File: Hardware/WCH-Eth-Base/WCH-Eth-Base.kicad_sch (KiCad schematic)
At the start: 1 part, among them J7 Conn_02x32_Counter_Clockwise

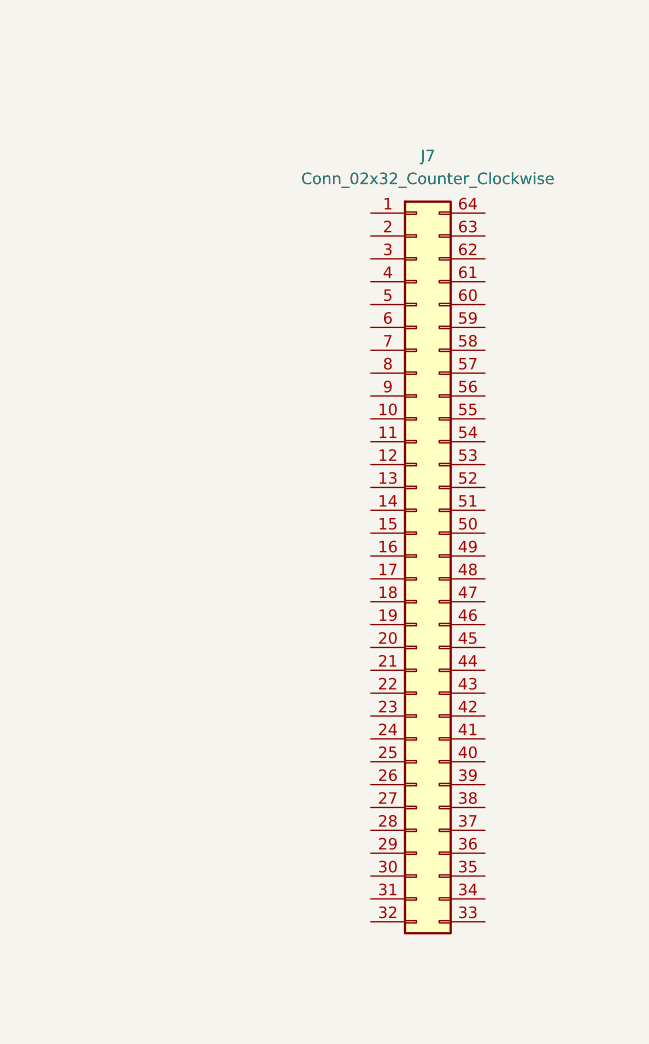
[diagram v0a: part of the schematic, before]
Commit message: add Files and First Layout things
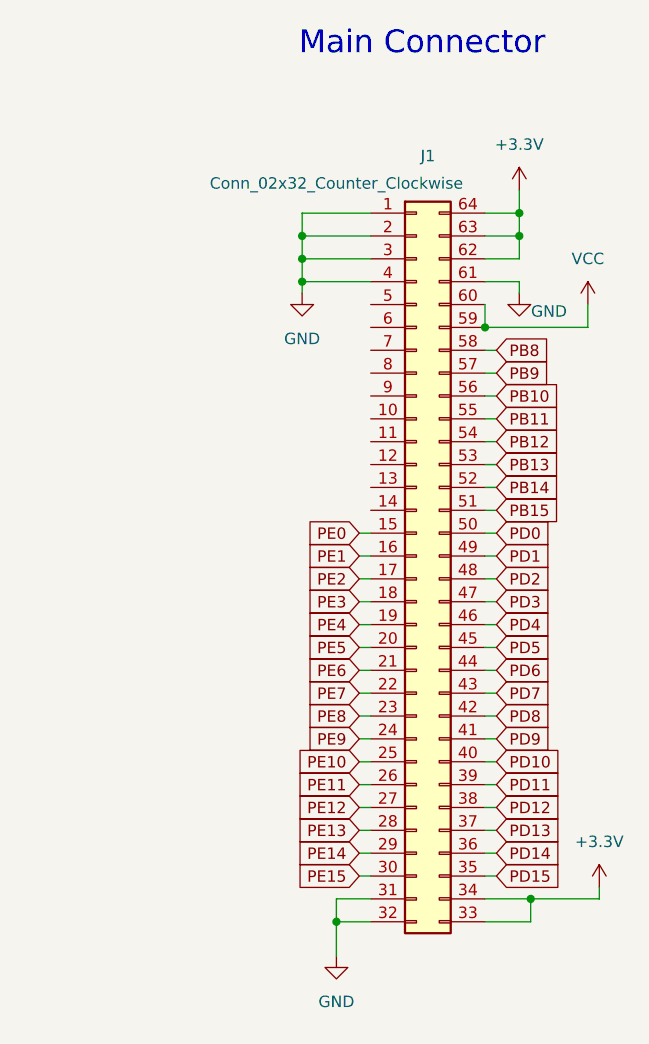
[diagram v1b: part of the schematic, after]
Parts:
- renumbered J7 to J1
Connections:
- net GND: now reaches J1.1 (Pin_1)
- net GND: now also J1.2 (Pin_2), J1.3 (Pin_3), J1.31 (Pin_31), J1.32 (Pin_32), J1.4 (Pin_4), J1.61 (Pin_61)
- net PE0: now reaches J1.15 (Pin_15)
- net PE1: now reaches J1.16 (Pin_16)
- net PE2: now reaches J1.17 (Pin_17)
- net PE3: now reaches J1.18 (Pin_18)
- net PE4: now reaches J1.19 (Pin_19)
- net PE5: now reaches J1.20 (Pin_20)
- net PE6: now reaches J1.21 (Pin_21)
- net PE7: now reaches J1.22 (Pin_22)
- net PE8: now reaches J1.23 (Pin_23)
- net PE9: now reaches J1.24 (Pin_24)
- net PE10: now reaches J1.25 (Pin_25)
- net PE11: now reaches J1.26 (Pin_26)
- net PE12: now reaches J1.27 (Pin_27)
- net PE13: now reaches J1.28 (Pin_28)
- net PE14: now reaches J1.29 (Pin_29)
- net PE15: now reaches J1.30 (Pin_30)
- net +3.3V: now reaches J1.33 (Pin_33)
- net +3.3V: now also J1.34 (Pin_34), J1.62 (Pin_62), J1.63 (Pin_63), J1.64 (Pin_64)
- net PD15: now reaches J1.35 (Pin_35)
- net PD14: now reaches J1.36 (Pin_36)
- net PD13: now reaches J1.37 (Pin_37)
- net PD12: now reaches J1.38 (Pin_38)
- net PD11: now reaches J1.39 (Pin_39)
- net PD10: now reaches J1.40 (Pin_40)
- net PD9: now reaches J1.41 (Pin_41)
- net PD8: now reaches J1.42 (Pin_42)
- net PD7: now reaches J1.43 (Pin_43)
- net PD6: now reaches J1.44 (Pin_44)
- net PD5: now reaches J1.45 (Pin_45)
- net PD4: now reaches J1.46 (Pin_46)
- net PD3: now reaches J1.47 (Pin_47)
- net PD2: now reaches J1.48 (Pin_48)
- net PD1: now reaches J1.49 (Pin_49)
- net PD0: now reaches J1.50 (Pin_50)
- net PB15: now reaches J1.51 (Pin_51)
- net PB14: now reaches J1.52 (Pin_52)
- net PB13: now reaches J1.53 (Pin_53)
- net PB12: now reaches J1.54 (Pin_54)
- net PB11: now reaches J1.55 (Pin_55)
- net PB10: now reaches J1.56 (Pin_56)
- net PB9: now reaches J1.57 (Pin_57)
- net PB8: now reaches J1.58 (Pin_58)
- net VCC: now reaches J1.59 (Pin_59)
- net VCC: now also J1.60 (Pin_60)
